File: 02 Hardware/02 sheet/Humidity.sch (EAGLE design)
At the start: 19 parts, among them IC1 IRM-03, IC2 Amica Modul V2 ESP8266 ESP-12F, J1 AC 230V, J2 Fan, J3 AM2302_OUT, J4 AM2302_IN, K1 351, Q1 BC817

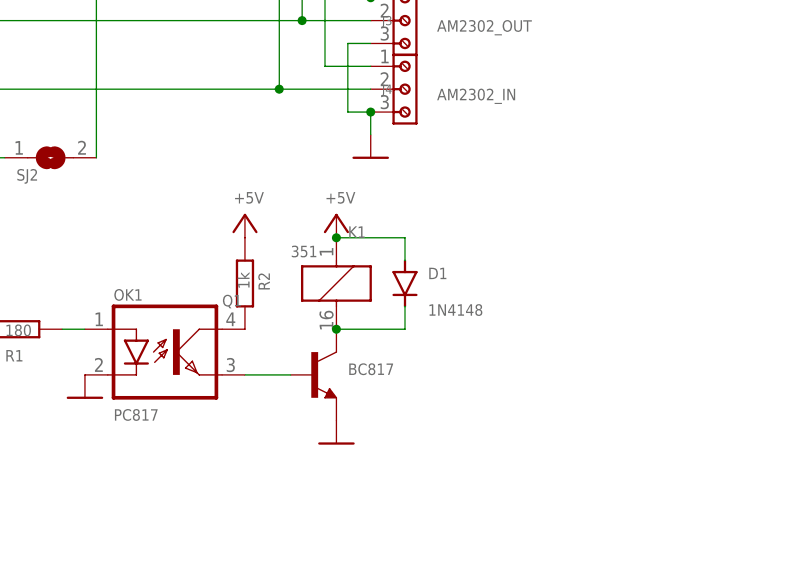
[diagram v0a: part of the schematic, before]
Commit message: Schaltung
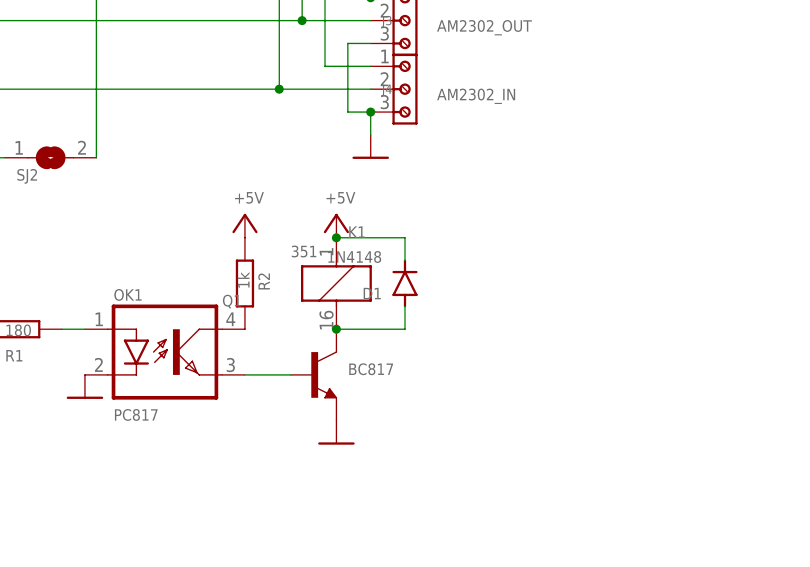
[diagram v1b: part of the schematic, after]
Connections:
- net +5V: now also D1.C; no longer D1.A
- net N$8: now also D1.A; no longer D1.C
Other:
- moved on the sheet: D1
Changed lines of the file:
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@@
 <layer number="91" name="Nets" color="2" fill="1" visible="yes" active="yes"/>
 <layer number="92" name="Busses" color="1" fill="1" visible="yes" active="yes"/>
-<layer number="93" name="Pins" color="2" fill="1" visible="no" active="yes"/>
+<layer number="93" name="Pins" color="2" fill="1" visible="yes" active="yes"/>
 <layer number="94" name="Symbols" color="4" fill="1" visible="yes" active="yes"/>
 <layer number="95" name="Names" color="7" fill="1" visible="yes" active="yes"/>
@@
 </instance>
 <instance part="GND4" gate="1" x="173.99" y="67.31" smashed="yes"/>
-<instance part="D1" gate="G$1" x="181.61" y="85.09" smashed="yes" rot="R270">
-<attribute name="NAME" x="184.15" y="85.5726" size="1.27" layer="95"/>
-<attribute name="VALUE" x="184.15" y="81.5086" size="1.27" layer="96"/>
+<instance part="D1" gate="G$1" x="181.61" y="85.09" smashed="yes" rot="R90">
+<attribute name="NAME" x="179.07" y="84.6074" size="1.27" layer="95" rot="R180"/>
+<attribute name="VALUE" x="179.07" y="88.6714" size="1.27" layer="96" rot="R180"/>
 </instance>
 <instance part="P+3" gate="1" x="120.65" y="49.53" smashed="yes">
@@
 <wire x1="173.99" y1="90.17" x2="181.61" y2="90.17" width="0.1524" layer="91"/>
 <junction x="173.99" y="90.17"/>
-<pinref part="D1" gate="G$1" pin="A"/>
-<wire x1="181.61" y1="90.17" x2="181.61" y2="87.63" width="0.1524" layer="91"/>
+<pinref part="D1" gate="G$1" pin="C"/>
+<wire x1="181.61" y1="87.63" x2="181.61" y2="90.17" width="0.1524" layer="91"/>
 </segment>
 <segment>
@@
 <wire x1="173.99" y1="80.01" x2="181.61" y2="80.01" width="0.1524" layer="91"/>
 <junction x="173.99" y="80.01"/>
-<pinref part="D1" gate="G$1" pin="C"/>
-<wire x1="181.61" y1="80.01" x2="181.61" y2="82.55" width="0.1524" layer="91"/>
-</segment>
-</net>
+<pinref part="D1" gate="G$1" pin="A"/>
+<wire x1="181.61" y1="82.55" x2="181.61" y2="80.01" width="0.1524" layer="91"/>
+</segment>
+</net>
